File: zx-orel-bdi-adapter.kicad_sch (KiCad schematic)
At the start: 31 parts, among them J1 Barrel_Jack_Switch, J2 DB9_Male, SW1 SW_Push_Dual, SW2 SW_DPDT_x2, U1 74LS30, U2 74LS27, U3 74LS04, U4 74LS640, U5 28C256

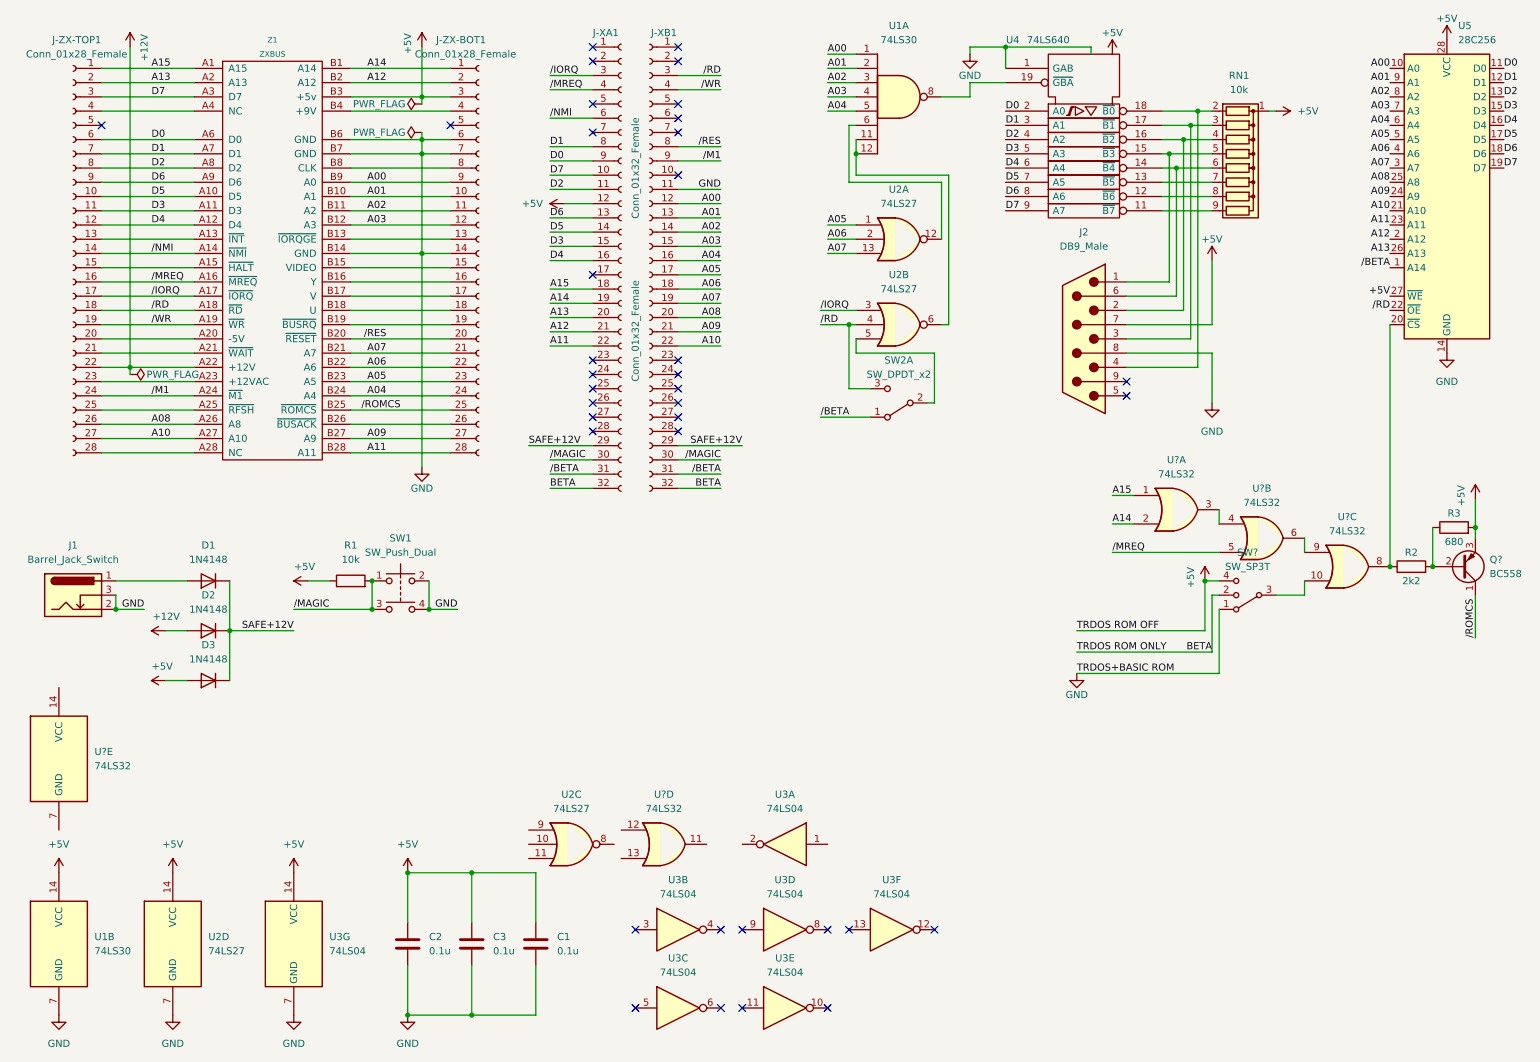
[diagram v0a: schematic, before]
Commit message: finished orel bdi to zxbus design
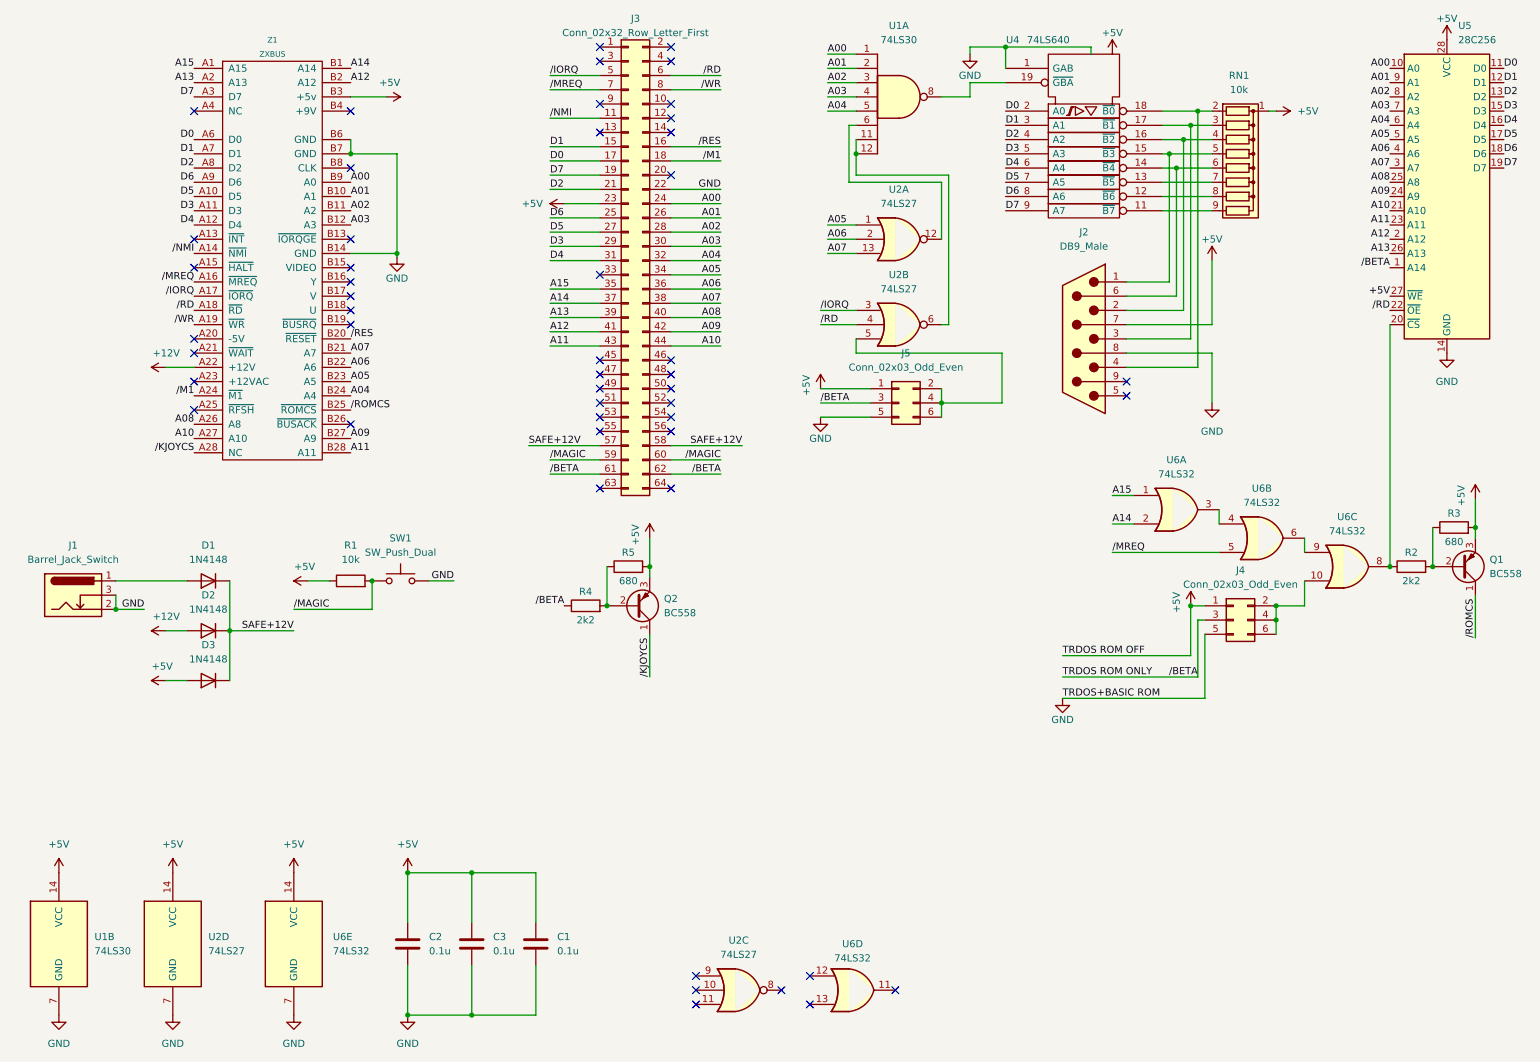
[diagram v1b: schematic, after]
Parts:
- removed J-XA1, J-XB1: Conn_01x32_Female, Connector_PinSocket_2.54mm:PinSocket_1x32_P2.54mm_Vertical, symbol Connector:Conn_01x32_Female
- removed J-ZX-BOT1, J-ZX-TOP1: Conn_01x28_Female, Connector_PinSocket_2.54mm:PinSocket_1x28_P2.54mm_Vertical, symbol Connector:Conn_01x28_Female
- removed SW2: SW_DPDT_x2, Button_Switch_THT:SW_NKK_G1xJP, symbol Switch:SW_DPDT_x2
- removed SW?: SW_SP3T, symbol Switch:SW_SP3T
- removed U3: 74LS04, Package_DIP:DIP-14_W7.62mm, symbol 74xx:74LS04
- removed U?: 74LS32, symbol 74xx:74LS32
- added J3: Conn_02x32_Row_Letter_First, Connector_PinHeader_2.54mm:PinHeader_2x32_P2.54mm_Vertical, symbol Connector_Generic:Conn_02x32_Odd_Even
- added J4, J5: Conn_02x03_Odd_Even, Connector_PinHeader_2.54mm:PinHeader_2x03_P2.54mm_Vertical, symbol Connector_Generic:Conn_02x03_Odd_Even
- added Q2: BC558, Package_TO_SOT_THT:TO-92_Inline_Wide, symbol Transistor_BJT:BC558
- added R4: 2k2, Resistor_THT:R_Axial_DIN0207_L6.3mm_D2.5mm_P7.62mm_Horizontal, symbol Device:R
- added R5: 680, Resistor_THT:R_Axial_DIN0207_L6.3mm_D2.5mm_P7.62mm_Horizontal, symbol Device:R
- added unit 4 of U6
- Q1: renamed from Q?; footprint Package_TO_SOT_THT:TO-92_Inline -> Package_TO_SOT_THT:TO-92_Inline_Wide
- R2, R3: footprint (none) -> Resistor_THT:R_Axial_DIN0207_L6.3mm_D2.5mm_P7.62mm_Horizontal
- SW1: symbol Switch:SW_Push_Dual -> Switch:SW_Push
- U6: renamed from U?; footprint (none) -> Package_DIP:DIP-14_W7.62mm
- Z1: footprint (none) -> RobikBUS:ZXBUS Slot Connector
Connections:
- net +5V: now also U6.14 (VCC), J3.23 (Pin_23), J4.1 (Pin_1), J5.1 (Pin_1), Q2.3 (E), R5.2
- net A00: now also J3.24 (Pin_24)
- net A01: now also J3.26 (Pin_26)
- net A02: now also J3.28 (Pin_28)
- net A03: now also J3.30 (Pin_30)
- net A04: now also J3.32 (Pin_32)
- net A05: now also J3.34 (Pin_34)
- net A06: now also J3.36 (Pin_36)
- net A07: now also J3.38 (Pin_38)
- net A08: now also J3.40 (Pin_40)
- net A09: now also J3.42 (Pin_42)
- net A10: now also J3.44 (Pin_44)
- net A11: now also J3.43 (Pin_43)
- net A12: now also J3.41 (Pin_41)
- net A13: now also J3.39 (Pin_39)
- net A14: now also J3.37 (Pin_37)
- net A15: now also J3.35 (Pin_35)
- net D0: now also J3.17 (Pin_17)
- net D1: now also J3.15 (Pin_15)
- net D2: now also J3.21 (Pin_21)
- net D3: now also J3.29 (Pin_29)
- net D4: now also J3.31 (Pin_31)
- net D5: now also J3.27 (Pin_27)
- net D6: now also J3.25 (Pin_25)
- net D7: now also J3.19 (Pin_19)
- net GND: now also U6.7 (GND), J3.22 (Pin_22), J4.5 (Pin_5), J5.5 (Pin_5); no longer SW1.4
- net SAFE+12V: now also J3.57 (Pin_57), J3.58 (Pin_58)
- net /IORQ: now also J3.5 (Pin_5)
- net /M1: now also J3.18 (Pin_18)
- net /MAGIC: now also J3.59 (Pin_59), J3.60 (Pin_60); no longer SW1.3
- net /MREQ: now also J3.7 (Pin_7)
- net /NMI: now also J3.11 (Pin_11)
- net /RD: now also J3.6 (Pin_6)
- net /RES: now also J3.16 (Pin_16)
- net /WR: now also J3.8 (Pin_8)
- net at U2.5: now also J5.2 (Pin_2), J5.4 (Pin_4), J5.6 (Pin_6)
- net at U6.10: now also J4.2 (Pin_2), J4.4 (Pin_4), J4.6 (Pin_6)
- net /KJOYCS: now reaches Z1.A28 (NC)
- net /KJOYCS: now also Q2.1 (C)
- net /BETA renamed TRDOS ROM ONLY
- net TRDOS ROM ONLY: now also J3.61 (Pin_61), J3.62 (Pin_62), J4.3 (Pin_3), J5.3 (Pin_3), R4.1
- new net: Q2.2 (B), R4.2, R5.1
- no-connect marks 37 -> 50
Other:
- moved on the sheet: U2C
